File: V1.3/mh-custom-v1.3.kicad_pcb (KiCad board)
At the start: 2 copper layers, 13 x 1.4 mm, 121 parts, among them J1 Conn_01x03_Male, J10 Screw_Terminal_01x02, J11 Screw_Terminal_01x02, J12 Screw_Terminal_01x02, J13 USB_A, J14 Screw_Terminal_01x02, J3 Conn_02x19_Top_Bottom, J4 Conn_02x19_Top_Bottom, J5 Screw_Terminal_01x02, J6 Screw_Terminal_01x02, J7 Screw_Terminal_01x02, J8 Screw_Terminal_01x02, J9 Screw_Terminal_01x02, SW1 SW_DIP_x04, T1 AO3400A, T2 AO3400A, T3 AO3400A, T4 AO3400A, T5 AO3400A, T6 AO3400A, U2 ADE7953xCP, U3 AMS1117-3.3, Y1 3.58MHz

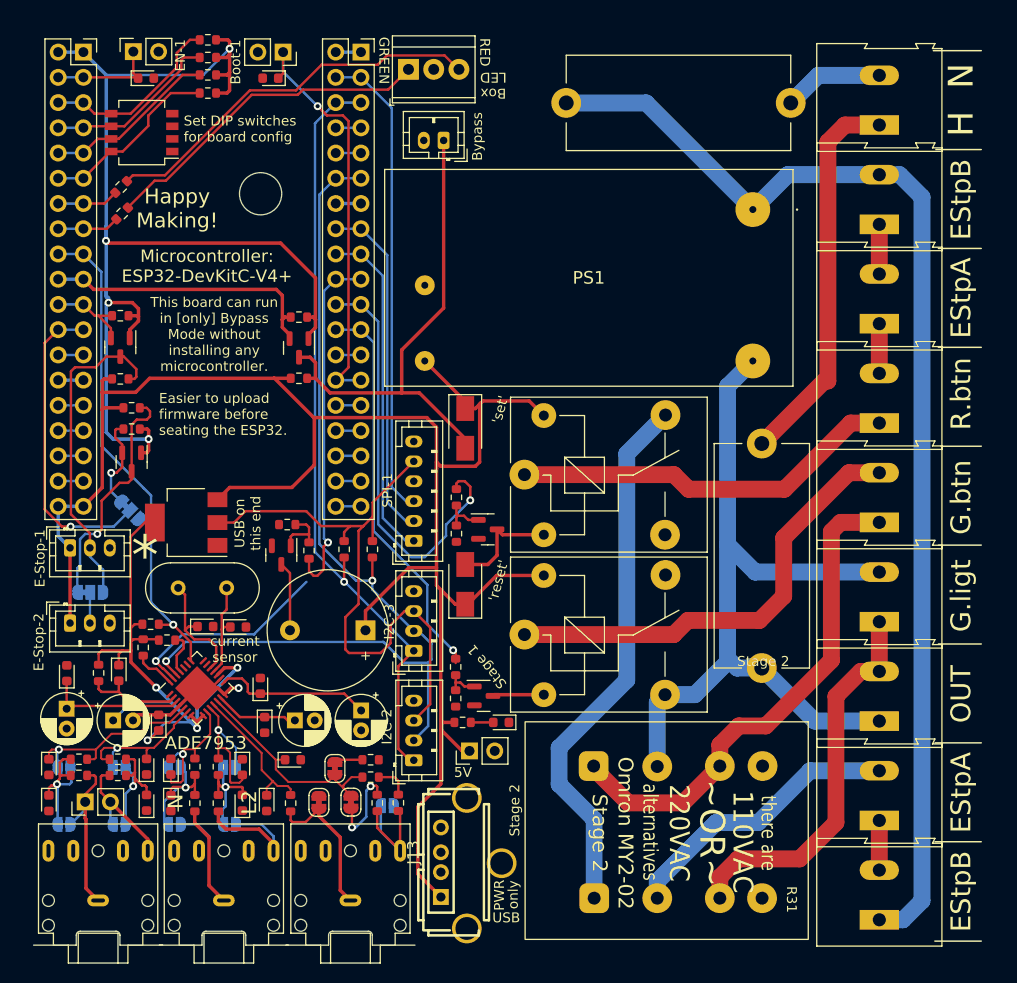
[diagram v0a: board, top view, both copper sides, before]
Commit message: fixing edges and connecting all pieces
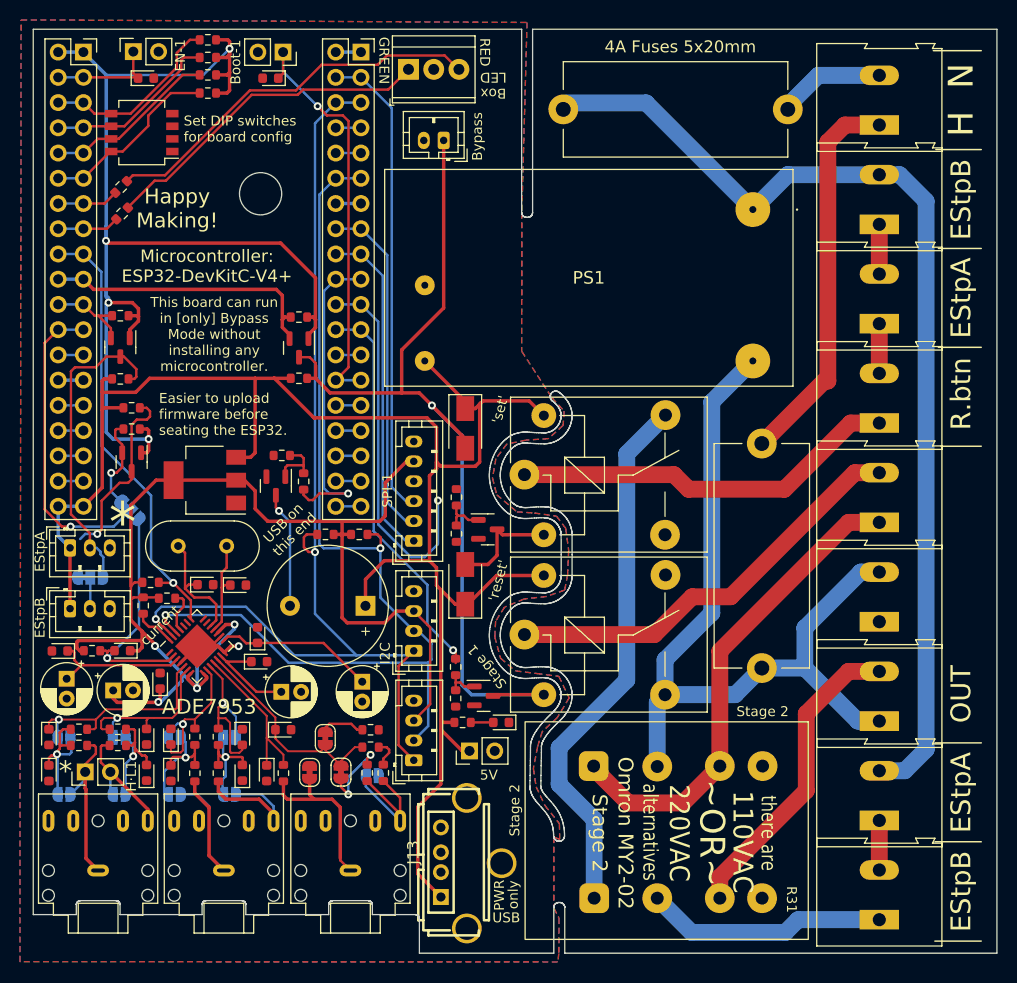
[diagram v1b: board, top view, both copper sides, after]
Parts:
- moved R1 6.98 mm to (60.2, 68.3)
- moved R2 6.98 mm to (58.0, 65.7)
- moved T1 6.98 mm to (57.4, 68.8)
- moved C22 6.39 mm to (55.7, 86.5), turned to 0 degrees
- moved C17 5.11 mm to (55.5, 83.8)
- moved U3 4.66 mm to (50.2, 68.2)
- moved C21 4.22 mm to (53.6, 78.8)
- moved C20 4.22 mm to (50.3, 78.7)
- moved R23 4.22 mm to (44.8, 78.5)
- moved R24 4.22 mm to (44.0, 80.8)
- moved R25 4.22 mm to (46.4, 80.1)
- moved U2 4.22 mm to (49.4, 84.9)
- moved Y1 4.22 mm to (52.4, 74.8)
- moved C13 4.21 mm to (45.7, 88.4)
- moved R13 3.38 mm to (68.2, 97.7)
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- renumbered E-Stop-1 to EStpA, E-Stop-2 to EStpB
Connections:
- J10 pad 2: Member-E-Stop-sw1-1 -> Member-E-Stop-aux2-2
- J11 pad 1: Member-E-Stop-aux2-2 -> Member-E-Stop-sw1-1
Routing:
- net read-bypass: track 55.2 -> 93.2 mm, vias 0 -> 1
- net Member-E-Stop-aux2-2: track 118.6 -> 104.0 mm
- net Net-(C15-Pad2): track 10.1 -> 24.5 mm, vias 0 -> 1
- net SCL: track 98.7 -> 108.0 mm
- net Green-Indicator-light-2: track 40.2 -> 31.3 mm
- net +5V: track 189.9 -> 181.6 mm
- net Net-(JP14-Pad1): track 24.2 -> 18.8 mm
- net GND: track 22.9 -> 17.5 mm
- net reset3v: track 43.0 -> 37.7 mm
- net /microcontroller/lightsounds/dcp1: track 6.99 -> 11.7 mm, vias 0 -> 1
- net Member-E-Stop-sw1-1: track 28.7 -> 24.3 mm
- net ade7953-IRQ: track 49.5 -> 45.2 mm
- net +3.3V: track 126.4 -> 130.3 mm
- net buzz: track 35.8 -> 32.2 mm
- net SDA: track 98.7 -> 102.2 mm
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- added copper zone on B.Cu, net GND
- added copper zone on F.Cu, net GND
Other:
- board size 13 x 1.4 mm -> 97 x 93 mm
- board text added: "4A Fuses 5x20mm"
- board text added: "H·L1"
- board text added: "I2C"
- board text added: "NEU/L2"
- board text added: "Volts"
- board text added: "current"
- board text removed: "G.btn"
- board text removed: "G.ligt"
- board text removed: "L2"
- board text removed: "current sensor"
- board text removed: "makehaven.org/toolauth"

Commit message: connections made, style points added. needs double-check
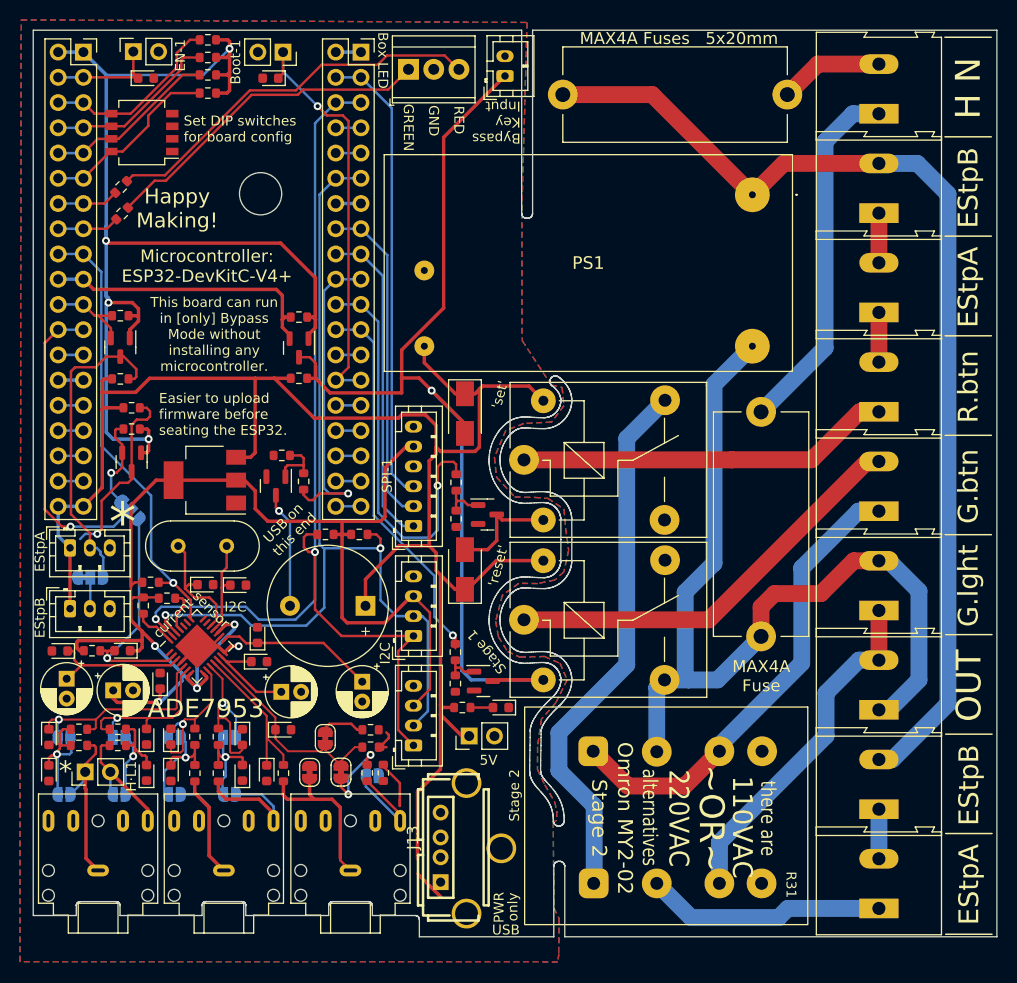
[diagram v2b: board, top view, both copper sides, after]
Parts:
- moved Bypass-1 10.4 mm to (80.9, 26.5), turned to 90 degrees
- moved F1 3.19 mm to (106.2, 72.8)
- moved D2 1.50 mm to (80.0, 91.1)
- moved D3 1.50 mm to (76.4, 61.5)
- moved D4 1.50 mm to (76.4, 77.2)
- moved I2C-2 1.50 mm to (71.2, 94.9)
- moved I2C-3 1.50 mm to (71.2, 83.9)
- moved J13 1.50 mm to (75.9, 105.2)
- moved R26 1.50 mm to (76.1, 91.1)
- moved R27 1.50 mm to (75.4, 85.5)
- moved R28 1.50 mm to (75.4, 88.7)
- moved R29 1.50 mm to (75.5, 68.4)
- moved T4 1.50 mm to (78.7, 71.7)
- moved R30 1.50 mm to (75.5, 72.1)
- moved SPI-1 1.50 mm to (71.2, 72.8)
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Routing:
- net read-bypass: track 93.2 -> 102.3 mm
- net Green-Indicator-light-1: track 84.6 -> 91.9 mm
- net SDA: track 102.2 -> 96.3 mm
- net VP_IN: track 16.0 -> 10.7 mm
- net Net-(R13-Pad1): track 2.89 -> 8.27 mm
- net Green-Indicator-light-2: track 31.3 -> 35.3 mm
- net reset3v: track 37.7 -> 41.1 mm
- net H/L1: track 39.2 -> 36.5 mm
- net Member-E-Stop-aux2-2: track 104.0 -> 106.1 mm
- net +3.3V: track 130.3 -> 132.3 mm
- net set3v: track 40.1 -> 38.6 mm
- net Member-Red-Reset-Button-1: track 39.1 -> 37.7 mm
- net Member-Green-Button-2: track 48.9 -> 47.6 mm
- net +5V: track 181.6 -> 182.3 mm
- net PICO: track 47.1 -> 46.4 mm
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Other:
- board size 97 x 93 mm -> 97 x 91.3 mm
- board text added: "3 stages of relays ESP32 WiFi microcontroller 2x E-Stop Integration Current Sensor"
- board text added: "Bypass Key Input"
- board text added: "G.btn"
- board text added: "G.lght"
- board text added: "GND"
- board text added: "H N"
- board text added: "Hardware:"
- board text added: "MAX4A Fuse"
- board text added: "MAX4A Fuses 5x20mm"
- board text added: "USB PWR No Data"
- board text added: "V1.3.0"
- board text added: "for daughter boards only"
- board text added: "makehaven.org/toolauth"
- board text added: "sensor"
- board text removed: "3 stages or relays WiFi microcontroller E-Stop Integration Current Sensor"
- board text removed: "4A Fuses 5x20mm"
- board text removed: "Bypass"
- board text removed: "H"
- board text removed: "Hardware: V1.3.0"
- board text removed: "N"
